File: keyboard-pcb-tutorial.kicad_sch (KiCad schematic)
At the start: 24 parts, among them SW1 SW_Push, U1 ATmega32U4-A, Y1 16MHz

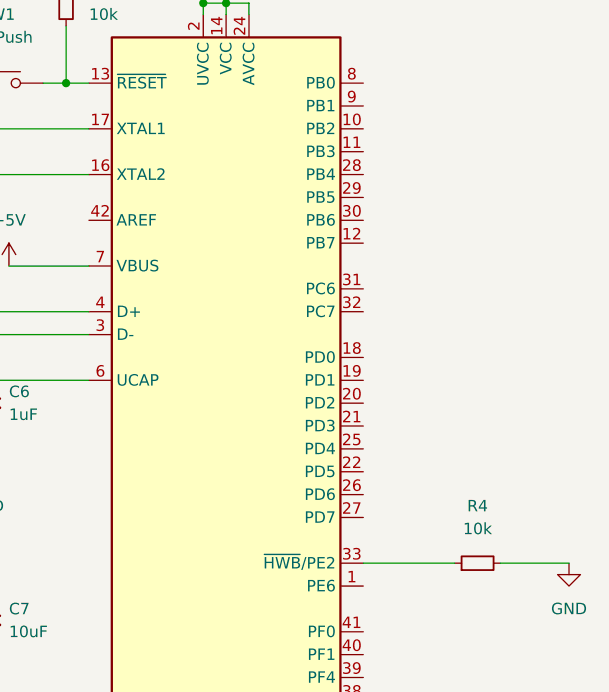
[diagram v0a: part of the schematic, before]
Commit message: Added routing
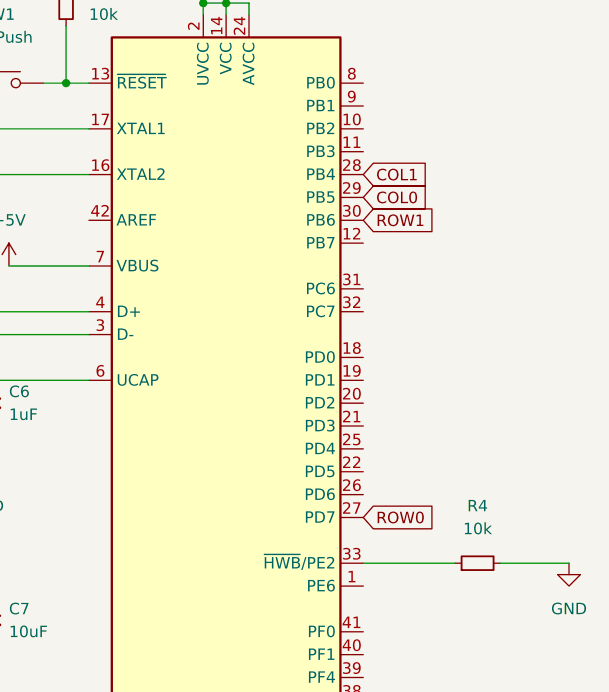
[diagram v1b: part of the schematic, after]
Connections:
- net COL0: now also U1.29 (PB5)
- net COL1: now also U1.28 (PB4)
- net ROW0: now also U1.27 (PD7)
- net ROW1: now also U1.30 (PB6)
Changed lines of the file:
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@@
     (stroke (width 0) (type default) (color 0 0 0 0))
+  )
+  (global_label "COL1" (shape input) (at 209.55 60.96 0) (fields_autoplaced)
+    (effects (font (size 1.27 1.27)) (justify left))
+    (property "Intersheet References" "${INTERSHEET_REFS}" (id 0) (at 216.8012 60.8806 0)
+      (effects (font (size 1.27 1.27)) (justify left) hide)
+    )
   )
   (global_label "ROW1" (shape input) (at 82.55 132.08 180) (fields_autoplaced)
@@
     )
   )
+  (global_label "COL0" (shape input) (at 209.55 63.5 0) (fields_autoplaced)
+    (effects (font (size 1.27 1.27)) (justify left))
+    (property "Intersheet References" "${INTERSHEET_REFS}" (id 0) (at 216.8012 63.4206 0)
+      (effects (font (size 1.27 1.27)) (justify left) hide)
+    )
+  )
+  (global_label "ROW1" (shape input) (at 209.55 66.04 0) (fields_autoplaced)
+    (effects (font (size 1.27 1.27)) (justify left))
+    (property "Intersheet References" "${INTERSHEET_REFS}" (id 0) (at 217.2245 65.9606 0)
+      (effects (font (size 1.27 1.27)) (justify left) hide)
+    )
+  )
   (global_label "ROW0" (shape input) (at 82.55 115.57 180) (fields_autoplaced)
     (effects (font (size 1.27 1.27)) (justify right))
@@
       (effects (font (size 1.27 1.27)) (justify left) hide)
     )
+  )
+  (global_label "ROW0" (shape input) (at 209.55 99.06 0) (fields_autoplaced)
+    (effects (font (size 1.27 1.27)) (justify left))
+    (property "Intersheet References" "${INTERSHEET_REFS}" (id 0) (at 217.2245 98.9806 0)
+      (effects (font (size 1.27 1.27)) (justify left) hide)
+    )
